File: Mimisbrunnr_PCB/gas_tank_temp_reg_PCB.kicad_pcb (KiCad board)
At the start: 2 copper layers, 118.8 x 56.6 mm, 43 parts, among them J1 Conn_01x04_Female, J10 Conn_01x06_Female, J2 Jack-DC, J3 Screw_Terminal_01x02, J4 Screw_Terminal_01x02, J5 Screw_Terminal_01x02, J6 Screw_Terminal_01x02, J7 Screw_Terminal_01x02, J8 Screw_Terminal_01x02, J9 Screw_Terminal_01x02, K1 SRD-12VDC-SL-C, K2 SRD-12VDC-SL-C, Q1 BC547, Q2 BC547, SW1 SW_Push, SW2 SW_Push, SW3 SW_Push, U1 ESP32-WROOM-32, U2 TLV76733DRVx, U3 MAX31856, U4 MAX31856, U5 MAX31856, U6 MAX31856, U7 MAX31856

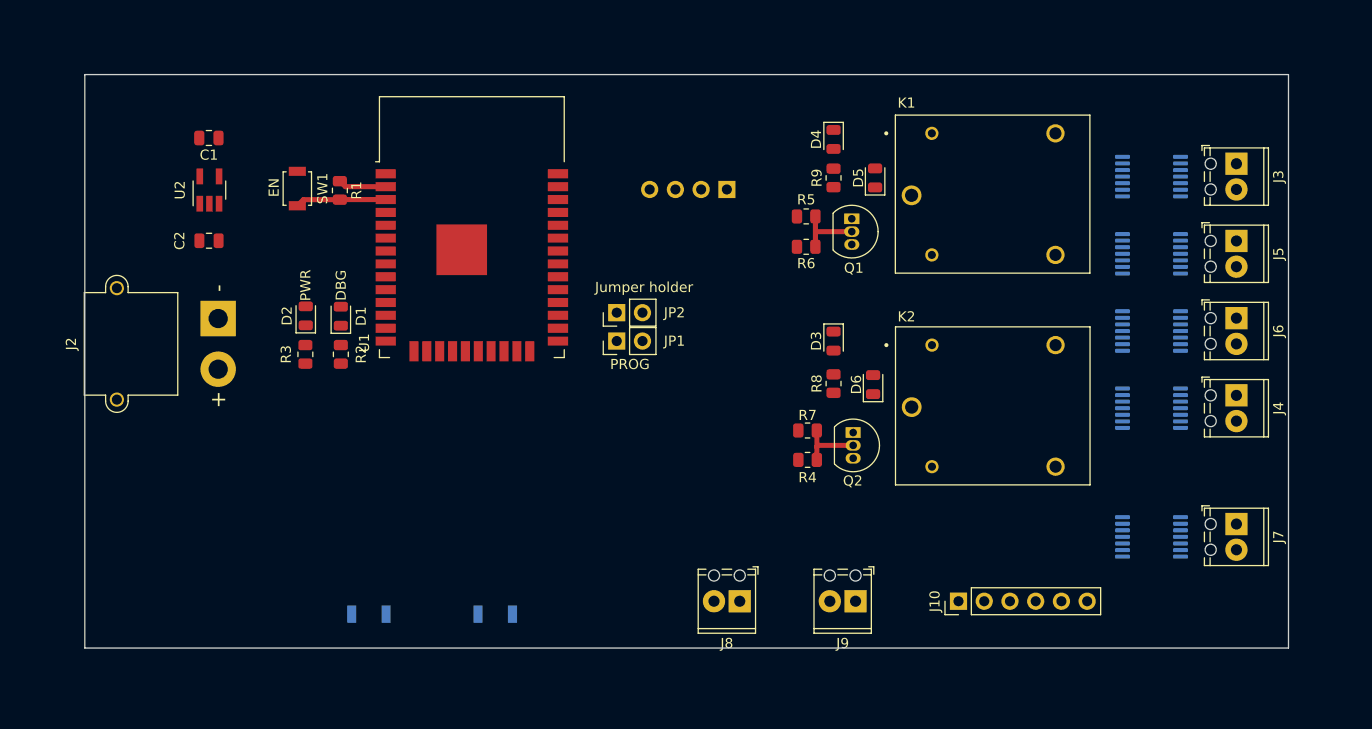
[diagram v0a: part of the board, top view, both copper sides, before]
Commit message: routing finished
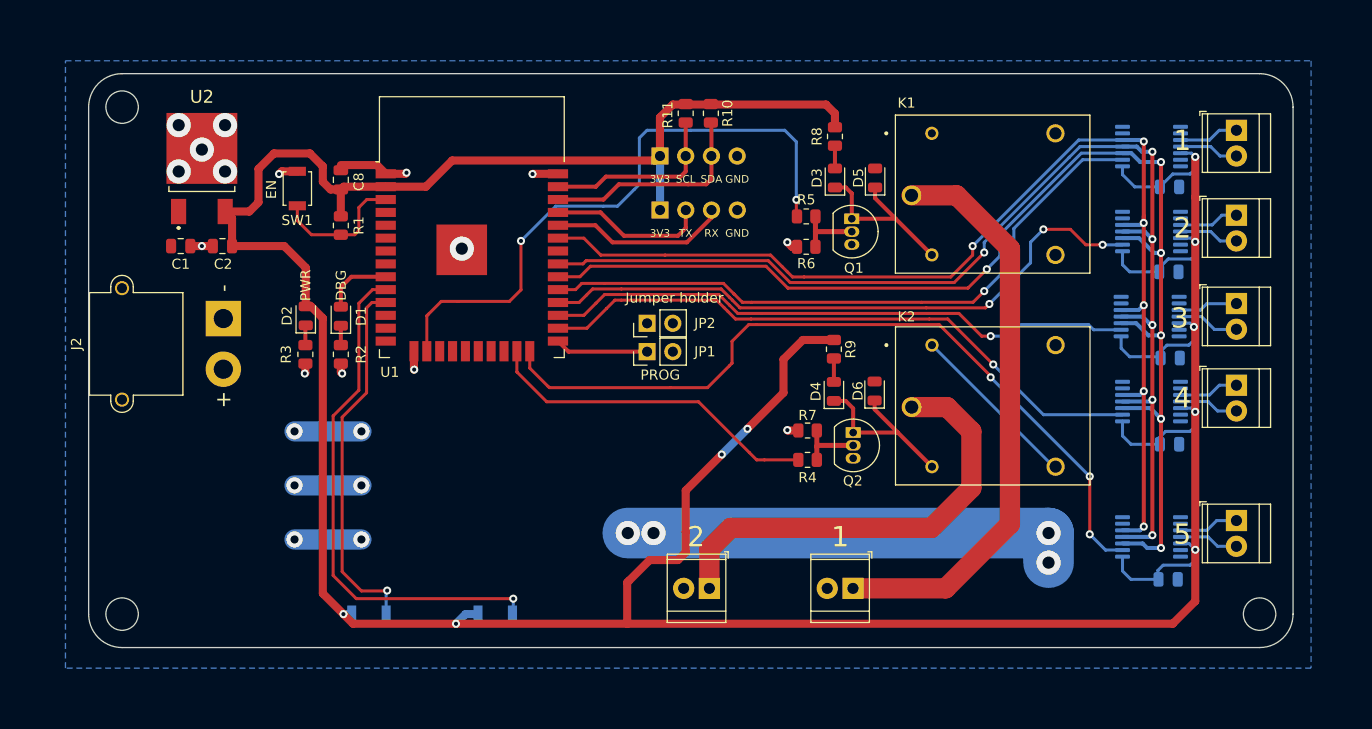
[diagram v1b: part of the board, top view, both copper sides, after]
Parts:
- added C3: C_Small, Capacitor_SMD:C_0805_2012Metric, B.Cu at (184.7, 91.2)
- added C4: C_Small, Capacitor_SMD:C_0805_2012Metric, B.Cu at (184.7, 65.8)
- added C5: C_Small, Capacitor_SMD:C_0805_2012Metric, B.Cu at (184.5, 104.5)
- added C6: C_Small, Capacitor_SMD:C_0805_2012Metric, B.Cu at (184.6, 74.2)
- added C7: C_Small, Capacitor_SMD:C_0805_2012Metric, B.Cu at (184.7, 82.7)
- added C8: C_Small, Capacitor_SMD:C_0805_2012Metric, F.Cu at (102.9, 65.1)
- added R10: 4k7, Resistor_SMD:R_0805_2012Metric, F.Cu at (139.4, 58.5)
- added R11: 4k7, Resistor_SMD:R_0805_2012Metric, F.Cu at (136.9, 58.5)
- added REF**: MountingHole_3.2mm_M3_ISO7380, MountingHole:MountingHole_3.2mm_M3_ISO7380, F.Cu at (193.5, 108.0)
- added REF**: MountingHole_3.2mm_M3_ISO7380, MountingHole:MountingHole_3.2mm_M3_ISO7380, F.Cu at (81.3, 108.0)
- added REF**: MountingHole_3.2mm_M3_ISO7380, MountingHole:MountingHole_3.2mm_M3_ISO7380, F.Cu at (81.3, 57.9)
- J10: value Conn_01x06_Female -> Conn_01x04_Female; footprint Connector_PinHeader_2.54mm:PinHeader_1x06_P2.54mm_Vertical -> Connector_PinHeader_2.54mm:PinHeader_1x04_P2.54mm_Vertical; moved to B.Cu
- J3, J4, J5, J6, J7, J8, J9: footprint TerminalBlock_Phoenix:TerminalBlock_Phoenix_MPT-0,5-2-2.54_1x02_P2.54mm_Horizontal -> TerminalBlock_TE-Connectivity:TerminalBlock_TE_282834-2_1x02_P2.54mm_Horizontal
- U2: value TLV76733DRVx -> BD733L5FP-CE2; footprint Package_TO_SOT_SMD:SOT-23-5_HandSoldering -> BD733L5FP:BD750L5FPCE2
- moved J10 48.6 mm to (134.4, 68.1), turned to -90 degrees
- moved D4 24.9 mm to (151.5, 86.0), turned to 90 degrees
- moved R8 24.4 mm to (151.6, 60.8), turned to -90 degrees
- moved R9 16.9 mm to (151.5, 81.8), turned to -90 degrees
- moved D3 16.1 mm to (151.6, 64.9), turned to 90 degrees
- moved J9 14.5 mm to (139.2, 105.4)
- moved J8 11.2 mm to (153.4, 105.4)
- moved C1 11.0 mm to (87.1, 71.6), turned to 0 degrees
- moved J1 7.38 mm to (134.4, 62.7), turned to -90 degrees
- moved U2 5.91 mm to (89.2, 60.2), turned to 0 degrees
- moved R1 3.46 mm to (102.9, 69.6)
- moved J3 3.30 mm to (191.3, 60.2)
- moved JP1 3.17 mm to (133.1, 82.0)
- moved JP2 3.17 mm to (133.1, 79.2)
- moved U3 2.96 mm to (182.9, 61.8)
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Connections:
- C2 pad 1: +3V3 -> +3.3V
- D2 pad 2: +3V3 -> +3.3V
- J1 pad 1: +3V3 -> +3.3V
- J1 pad 2: SDA -> SCL
- J1 pad 3: SCL -> SDA
- J10 pad 2: mosi -> ESP32_TX
- J10 pad 3: miso -> ESP32_RX
- J10 pad 4: sck -> GND
- J4 pad 1: tank_thc_2- -> tank_thc_4-
- J4 pad 2: tank_thc_2+ -> tank_thc_4+
- J5 pad 1: tank_thc_3- -> tank_thc_2-
- J5 pad 2: tank_thc_3+ -> tank_thc_2+
- J6 pad 1: tank_thc_4- -> tank_thc_3-
- J6 pad 2: tank_thc_4+ -> tank_thc_3+
- R1 pad 1: +3V3 -> +3.3V
- R8 pad 1: +3V3 -> +3.3V
- R9 pad 1: +3V3 -> +3.3V
- SW2 pad 2: +3V3 -> +3.3V
- SW3 pad 2: +3V3 -> +3.3V
- U1 pad 13: Relay2 -> unconnected-(U1-Pad13)
- U1 pad 16: Relay1 -> Relay1_CTRL
- U1 pad 2: +3V3 -> +3.3V
- U1 pad 23: unconnected-(U1-Pad23) -> Relay2_CTRL
- U1 pad 24: unconnected-(U1-Pad24) -> thc_water_cs
- U1 pad 26: thc1_cs -> thc4_cs
- U1 pad 27: thc2_cs -> thc3_cs
- U1 pad 28: thc3_cs -> thc2_cs
- U1 pad 29: thc4_cs -> thc1_cs
- U1 pad 33: unconnected-(U1-Pad33) -> mosi
- U1 pad 36: unconnected-(U1-Pad36) -> SDA
- U1 pad 37: mosi -> SCL
- U1 pad 8: thc_water_cs -> unconnected-(U1-Pad8)
- U2 pad 1: +3V3 -> +12V
- U2 pad 3: GND -> +3.3V
- U2 pad 4: +12V -> GND
- U3 pad 1: Earth -> GND
- U3 pad 14: Earth -> GND
- U3 pad 2: Earth -> GND
- U4 pad 1: Earth -> GND
- U4 pad 14: Earth -> GND
- U4 pad 2: Earth -> GND
- U4 pad 3: tank_thc_2- -> tank_thc_4-
- U4 pad 4: tank_thc_2+ -> tank_thc_4+
- U4 pad 9: thc2_cs -> thc4_cs
- U5 pad 1: Earth -> GND
- U5 pad 14: Earth -> GND
- U5 pad 2: Earth -> GND
- U5 pad 3: tank_thc_3- -> tank_thc_2-
- U5 pad 4: tank_thc_3+ -> tank_thc_2+
- U5 pad 9: thc3_cs -> thc2_cs
- U6 pad 1: Earth -> GND
- U6 pad 14: Earth -> GND
- U6 pad 2: Earth -> GND
- U6 pad 3: tank_thc_4- -> tank_thc_3-
- U6 pad 4: tank_thc_4+ -> tank_thc_3+
- U6 pad 9: thc4_cs -> thc3_cs
- U7 pad 1: Earth -> GND
- U7 pad 14: Earth -> GND
- U7 pad 2: Earth -> GND
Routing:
- net +3.3V: track 0.00 -> 366.2 mm, vias 0 -> 9
- net sck: track 0.00 -> 123.6 mm, vias 0 -> 6
- net miso: track 0.00 -> 116.9 mm, vias 0 -> 6
- net mosi: track 0.00 -> 113.4 mm, vias 0 -> 6
- net +12V: track 0.00 -> 81.4 mm, vias 0 -> 10
- net thc_water_cs: track 0.00 -> 77.4 mm, vias 0 -> 3
- net thc1_cs: track 0.00 -> 64.5 mm, vias 0 -> 1
- net thc2_cs: track 0.00 -> 62.1 mm, vias 0 -> 3
- net thc4_cs: track 0.00 -> 61.6 mm, vias 0 -> 1
- net Relay1_CTRL: track 0.00 -> 60.9 mm, vias 0 -> 2
- net thc3_cs: track 0.00 -> 58.8 mm, vias 0 -> 1
- net Relay1_conn: track 0.00 -> 57.2 mm
- net button-: track 0.00 -> 51.4 mm, vias 0 -> 1
- net Relay2_conn: track 0.00 -> 44.7 mm
- net button+: track 0.00 -> 36.8 mm, vias 0 -> 1
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- added copper zone on F.Cu, net +12V
- added copper zone on B.Cu, net GND
- removed copper zone on F.Cu, net GND
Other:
- board size 118.8 x 56.6 mm -> 118.9 x 56.6 mm
- board text added: "1"
- board text added: "2"
- board text added: "3"
- board text added: "3V3"
- board text added: "4"
- board text added: "5"
- board text added: "GND"
- board text added: "RX"
- board text added: "SCL"
- board text added: "SDA"
- board text added: "TX"
